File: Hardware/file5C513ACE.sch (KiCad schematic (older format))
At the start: 73 parts, among them J1 GATE_2, J2 GATE_3, J3 GATE_1, Q1 MMBT3904, Q2 MMBT3904, Q3 MMBT3904, SW1 Frequency Adjust, SW10 SET_SW, SW11 FILTER_SW, SW12 FILTEREXT_SW, SW13 SHAPE_SW, SW2 MOD_SW, SW3 FILTER1_SW, SW4 PROG, SW5 VOICE_SW, SW6 FILTER2_SW, SW7 RST, SW8 MODE_SW, SW9 FILTER3_SW, U1 TLC5947DAP

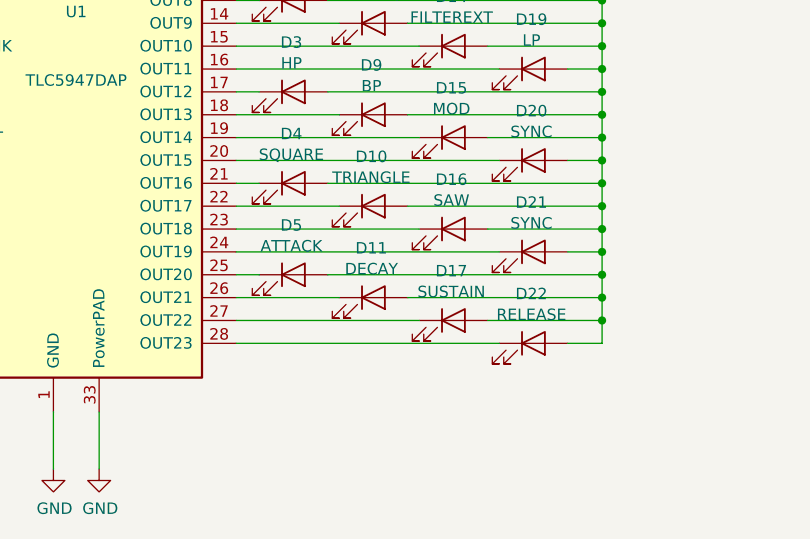
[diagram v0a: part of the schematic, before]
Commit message: Updated ADSR sliders
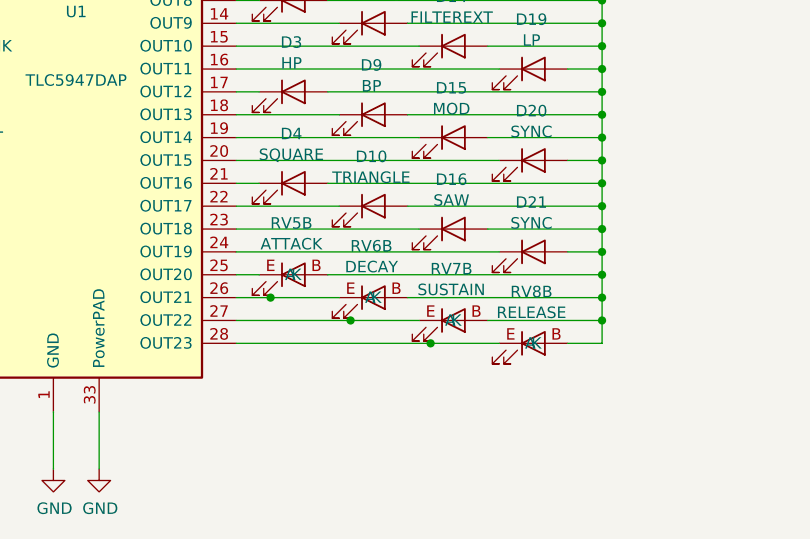
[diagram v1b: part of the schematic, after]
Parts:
- removed D11: DECAY, LED_THT:LED_D3.0mm, symbol Device:LED
- removed D17: SUSTAIN, LED_THT:LED_D3.0mm, symbol Device:LED
- removed D22: RELEASE, LED_THT:LED_D3.0mm, symbol Device:LED
- removed D5: ATTACK, LED_THT:LED_D3.0mm, symbol Device:LED
- added RV5: ATTACK, Potentiometer_THT:Potentiometer_Bourns_PTL20_Single_Slide, symbol SID_Parts:BOURNS_PTL
- added RV6: DECAY, Potentiometer_THT:Potentiometer_Bourns_PTL20_Single_Slide, symbol SID_Parts:BOURNS_PTL
- added RV7: SUSTAIN, Potentiometer_THT:Potentiometer_Bourns_PTL20_Single_Slide, symbol SID_Parts:BOURNS_PTL
- added RV8: RELEASE, Potentiometer_THT:Potentiometer_Bourns_PTL20_Single_Slide, symbol SID_Parts:BOURNS_PTL
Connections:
- net 3.3_IO: now also RV5.B (A), RV6.B (A), RV7.B (A), RV8.B (A)
- net at U1.25 (OUT20): now also RV5.E (K)
- net at U1.26 (OUT21): now also RV6.E (K)
- net at U1.27 (OUT22): now also RV7.E (K)
- net at U1.28 (OUT23): now also RV8.E (K)
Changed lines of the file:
@@
-	1    0    0    -1
-$EndComp
-$Comp
-L Device:LED D?
-U 1 1 5C6023D5
-P 2750 5550
-AR Path="/5BFD63E3/5C6023D5" Ref="D?"  Part="1"
-AR Path="/5BFD63E3/5C513ACF/5C6023D5" Ref="D5"  Part="1"
-F 0 "D5" H 2741 5766 50  0000 C CNN
-F 1 "ATTACK" H 2741 5675 50  0000 C CNN
-F 2 "LED_THT:LED_D3.0mm" H 2750 5550 50  0001 C CNN
-F 3 "~" H 2750 5550 50  0001 C CNN
-	1    2750 5550
-	1    0    0    -1
-$EndComp
-$Comp
-L Device:LED D?
-U 1 1 5C6023DC
-P 3100 5650
-AR Path="/5BFD63E3/5C6023DC" Ref="D?"  Part="1"
-AR Path="/5BFD63E3/5C513ACF/5C6023DC" Ref="D11"  Part="1"
-F 0 "D11" H 3091 5866 50  0000 C CNN
-F 1 "DECAY" H 3091 5775 50  0000 C CNN
-F 2 "LED_THT:LED_D3.0mm" H 3100 5650 50  0001 C CNN
-F 3 "~" H 3100 5650 50  0001 C CNN
-	1    3100 5650
-	1    0    0    -1
-$EndComp
-$Comp
-L Device:LED D?
-U 1 1 5C6023E3
-P 3450 5750
-AR Path="/5BFD63E3/5C6023E3" Ref="D?"  Part="1"
-AR Path="/5BFD63E3/5C513ACF/5C6023E3" Ref="D17"  Part="1"
-F 0 "D17" H 3441 5966 50  0000 C CNN
-F 1 "SUSTAIN" H 3441 5875 50  0000 C CNN
-F 2 "LED_THT:LED_D3.0mm" H 3450 5750 50  0001 C CNN
-F 3 "~" H 3450 5750 50  0001 C CNN
-	1    3450 5750
-	1    0    0    -1
-$EndComp
-$Comp
-L Device:LED D?
-U 1 1 5C6023EA
-P 3800 5850
-AR Path="/5BFD63E3/5C6023EA" Ref="D?"  Part="1"
-AR Path="/5BFD63E3/5C513ACF/5C6023EA" Ref="D22"  Part="1"
-F 0 "D22" H 3791 6066 50  0000 C CNN
-F 1 "RELEASE" H 3791 5975 50  0000 C CNN
-F 2 "LED_THT:LED_D3.0mm" H 3800 5850 50  0001 C CNN
-F 3 "~" H 3800 5850 50  0001 C CNN
-	1    3800 5850
 	1    0    0    -1
 $EndComp
@@
 	2500 5550 2600 5550
 Wire Wire Line
-	2500 5650 2950 5650
-Wire Wire Line
-	2500 5750 3300 5750
-Wire Wire Line
-	2500 5850 3650 5850
+	2500 5650 2650 5650
+Wire Wire Line
+	2500 5750 3000 5750
+Wire Wire Line
+	2500 5850 3350 5850
 Wire Wire Line
 	4100 3450 4100 3550
@@
 Text GLabel 4100 3450 1    50   Input ~ 0
 3.3_IO
+$Comp
+L SID_Parts:BOURNS_PTL RV?
+U 2 1 5C0B06A6
+P 2900 5500
+AR Path="/5BFD63E3/5C513EEB/5C0B06A6" Ref="RV?"  Part="2"
+AR Path="/5BFD63E3/5C513ACF/5C0B06A6" Ref="RV5"  Part="2"
+F 0 "RV5" V 2725 5341 50  0000 C CNN
+F 1 "ATTACK" V 2816 5341 50  0000 C CNN
+F 2 "Potentiometer_THT:Potentiometer_Bourns_PTL20_Single_Slide" H 2900 5500 50  0001 C CNN
+F 3 "" H 2900 5500 50  0001 C CNN
+	2    2900 5500
+	0    1    1    0
+$EndComp
+$Comp
+L SID_Parts:BOURNS_PTL RV?
+U 2 1 5C0B06AD
+P 3600 5700
+AR Path="/5BFD63E3/5C513EEB/5C0B06AD" Ref="RV?"  Part="2"
+AR Path="/5BFD63E3/5C513ACF/5C0B06AD" Ref="RV7"  Part="2"
+F 0 "RV7" V 3425 5541 50  0000 C CNN
+F 1 "SUSTAIN" V 3516 5541 50  0000 C CNN
+F 2 "Potentiometer_THT:Potentiometer_Bourns_PTL20_Single_Slide" H 3600 5700 50  0001 C CNN
+F 3 "" H 3600 5700 50  0001 C CNN
+	2    3600 5700
+	0    1    1    0
+$EndComp
+$Comp
+L SID_Parts:BOURNS_PTL RV?
+U 2 1 5C0B06B4
+P 3950 5800
+AR Path="/5BFD63E3/5C513EEB/5C0B06B4" Ref="RV?"  Part="2"
+AR Path="/5BFD63E3/5C513ACF/5C0B06B4" Ref="RV8"  Part="2"
+F 0 "RV8" V 3775 5641 50  0000 C CNN
+F 1 "RELEASE" V 3866 5641 50  0000 C CNN
+F 2 "Potentiometer_THT:Potentiometer_Bourns_PTL20_Single_Slide" H 3950 5800 50  0001 C CNN
+F 3 "" H 3950 5800 50  0001 C CNN
+	2    3950 5800
+	0    1    1    0
+$EndComp
+$Comp
+L SID_Parts:BOURNS_PTL RV?
+U 2 1 5C0B06BB
+P 3250 5600
+AR Path="/5BFD63E3/5C513EEB/5C0B06BB" Ref="RV?"  Part="2"
+AR Path="/5BFD63E3/5C513ACF/5C0B06BB" Ref="RV6"  Part="2"
+F 0 "RV6" V 3075 5441 50  0000 C CNN
+F 1 "DECAY" V 3166 5441 50  0000 C CNN
+F 2 "Potentiometer_THT:Potentiometer_Bourns_PTL20_Single_Slide" H 3250 5600 50  0001 C CNN
+F 3 "" H 3250 5600 50  0001 C CNN
+	2    3250 5600
+	0    1    1    0
+$EndComp
+Connection ~ 2650 5650
+Wire Wire Line
+	2650 5650 2950 5650
+Connection ~ 3000 5750
+Wire Wire Line
+	3000 5750 3300 5750
+Connection ~ 3350 5850
+Wire Wire Line
+	3350 5850 3650 5850
 $EndSCHEMATC
